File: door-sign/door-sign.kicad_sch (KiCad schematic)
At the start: 7 parts, among them SW1 200MSP1T1B1M2QEH

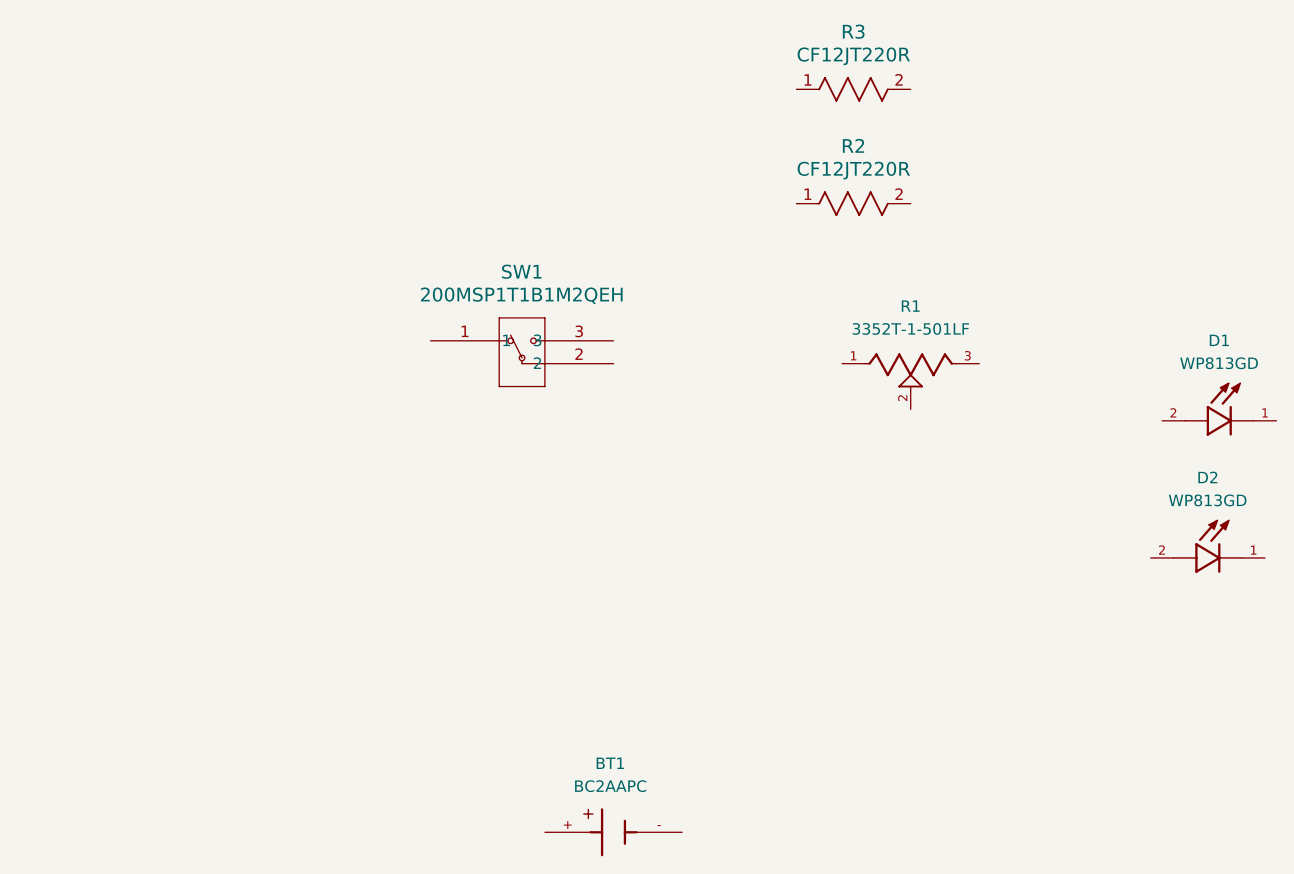
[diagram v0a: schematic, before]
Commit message: changed design
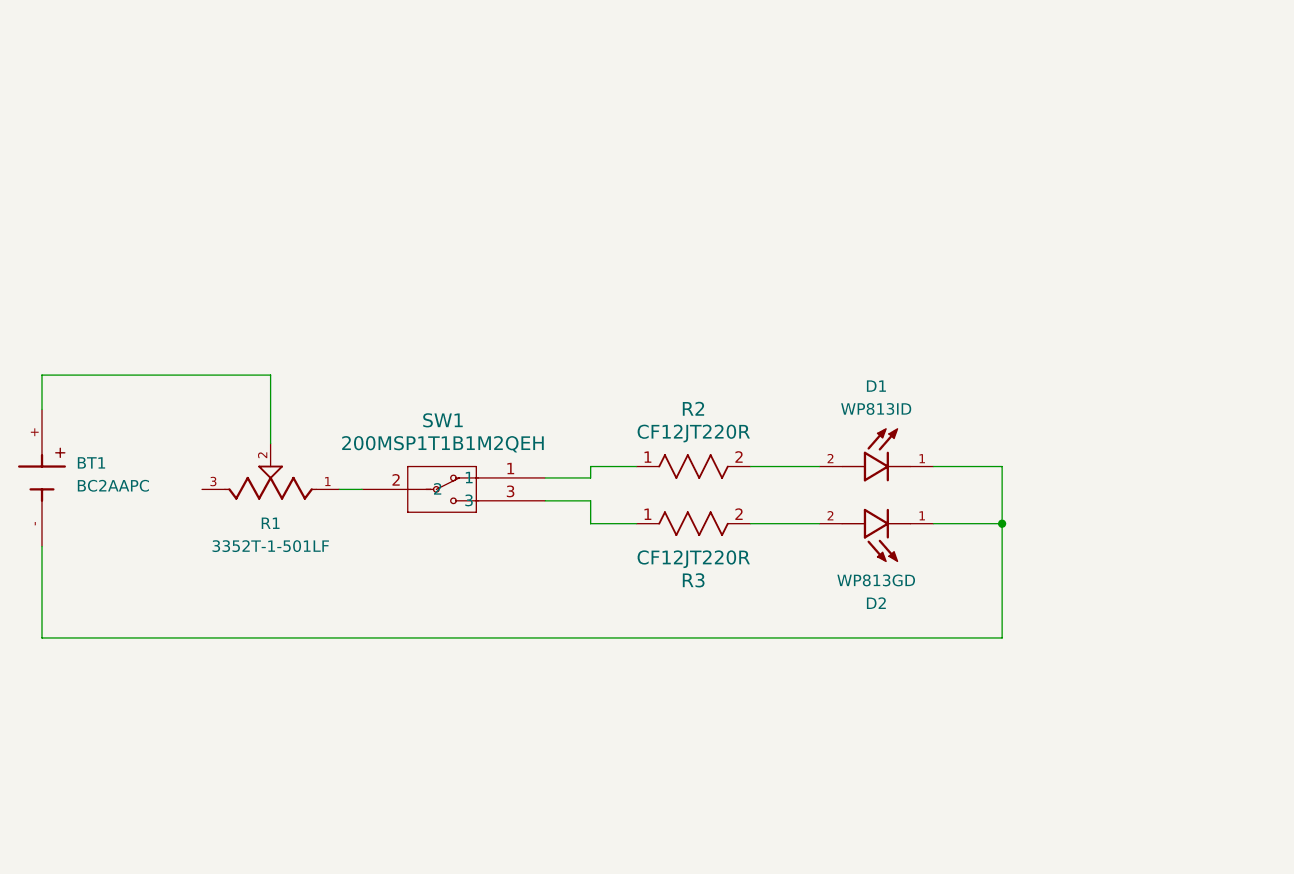
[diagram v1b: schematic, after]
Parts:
- D1: value WP813GD -> WP813ID
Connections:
- net at BT1.+: now also R1.2
- net at BT1.-: now also D1.1, D2.1
- net at D1.2: now also R2.2
- net at R2.1: now also SW1.1
- net at SW1.2: now also R1.1
- net at SW1.3: now also R3.1
- net at R3.2: now also D2.2
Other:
- moved on the sheet: BT1, D1, D2, R1, R2, R3, SW1
